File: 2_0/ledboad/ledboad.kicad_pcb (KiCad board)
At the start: 4 copper layers, 100 x 32 mm, 297 parts, among them J1 USB_C_Receptacle_USB2.0, Q10 CJX3139K, Q11 CJX3139K, Q12 CJX3139K, Q13 CJX3139K, Q14 CJX3139K, Q15 CJX3139K, Q16 CJX3139K, Q9 CJX3139K, SW2 TS-1088-AR02016, U2 74HC138PW,118

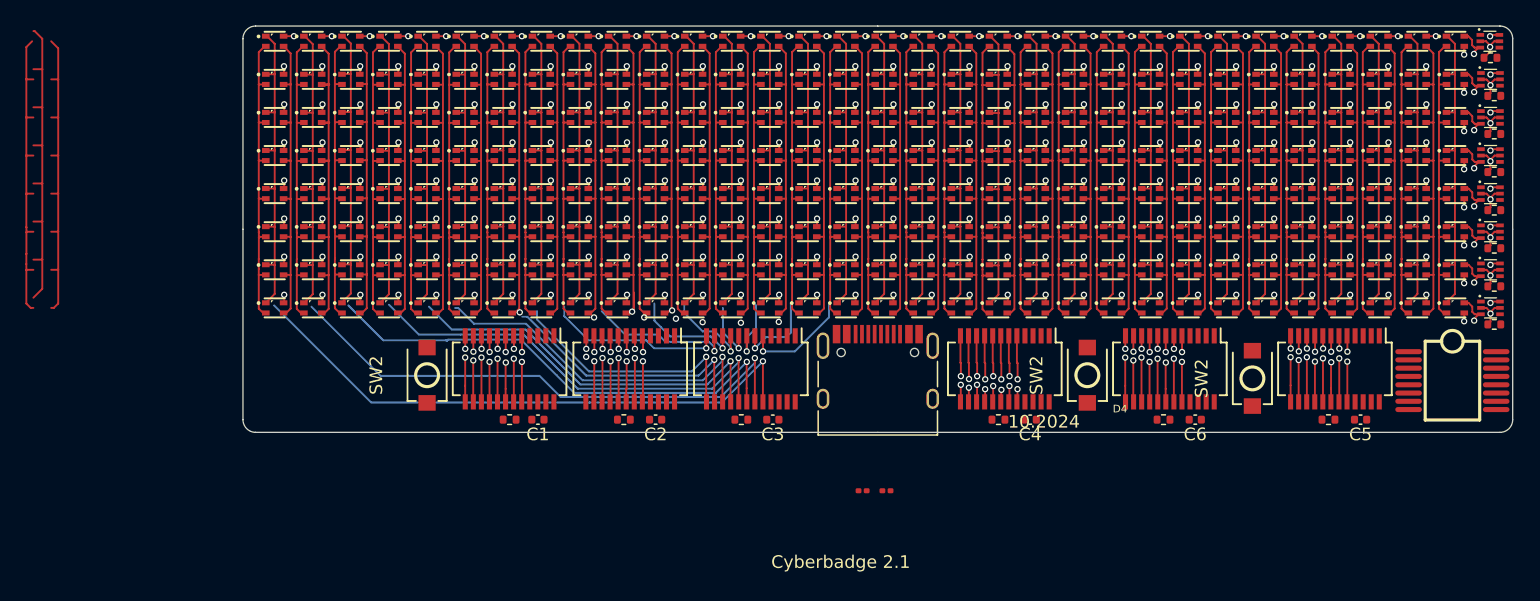
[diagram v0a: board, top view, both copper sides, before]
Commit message: work on ledboard
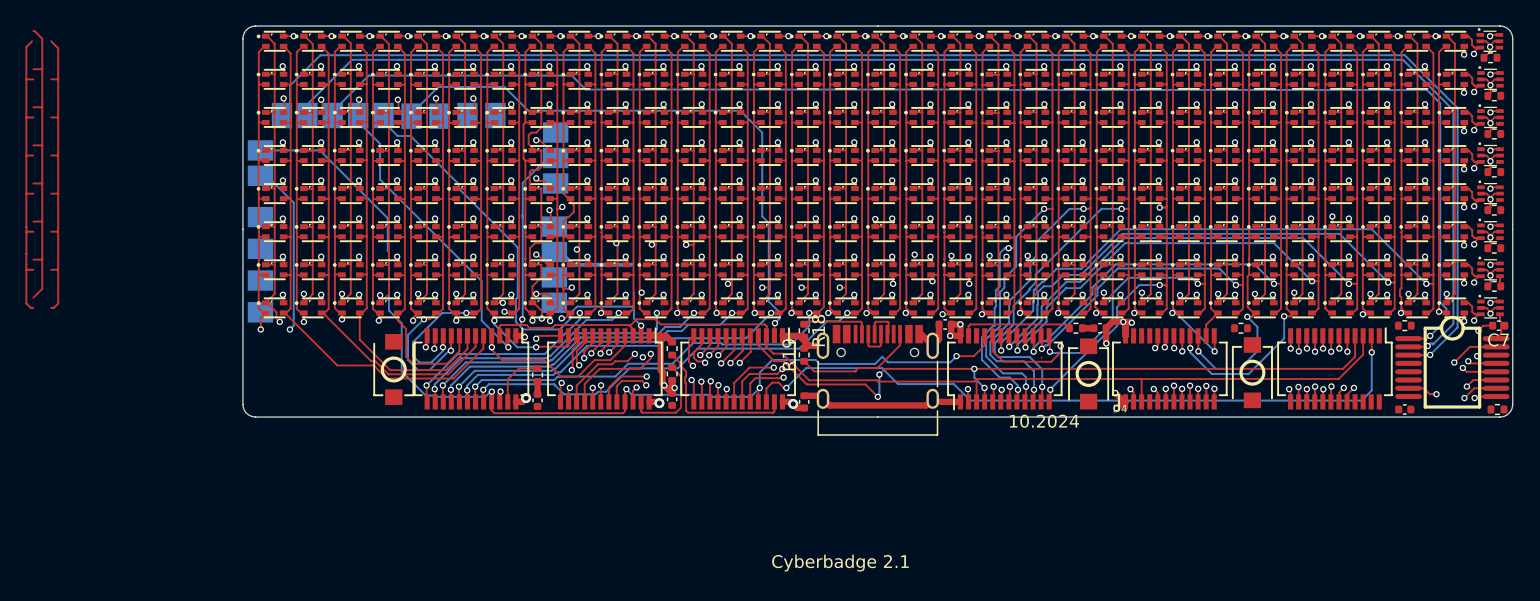
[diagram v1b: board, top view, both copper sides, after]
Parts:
- removed the SW2 at (54.5, 47.5)
- removed the SW2 at (119.5, 47.8)
- added C7: 470n, Capacitor_SMD:C_0402_1005Metric, F.Cu at (138.9, 43.6)
- added SW1: TS-1088-AR02016, easyeda2kicad:SW-SMD_L3.9-W3.0-P4.45, F.Cu at (119.5, 47.3)
- added SW3: TS-1088-AR02016, easyeda2kicad:SW-SMD_L3.9-W3.0-P4.45, F.Cu at (51.9, 47.0)
- added U1: ~, Critbit_lib:pilkbrain2, B.Cu at (53.4, 38.8)
- R18, R19: footprint Resistor_SMD:R_0201_0603Metric -> Resistor_SMD:R_0402_1005Metric
- moved C5 33.6 mm to (95.3, 43.5)
- moved C6 16.5 mm to (131.5, 50.2), turned to 0 degrees
- moved R18 14.2 mm to (84.2, 44.0), turned to -90 degrees
- moved R19 11.6 mm to (84.2, 45.9), turned to 90 degrees
- moved R9 9.53 mm to (131.5, 43.6)
- moved R11 9.44 mm to (118.6, 43.8)
- moved R13 9.44 mm to (105.6, 43.8)
- moved C4 9.06 mm to (107.5, 43.8)
- moved R10 7.81 mm to (73.8, 45.4), turned to 90 degrees
- moved R24 6.70 mm to (138.8, 50.2)
- moved R12 5.23 mm to (73.8, 47.4), turned to -90 degrees
- moved R14 4.15 mm to (63.2, 47.5), turned to -90 degrees
- moved RU6 3.00 mm to (58.0, 47.0)
- moved C3 2.84 mm to (84.2, 49.6), turned to 90 degrees
- moved C2 2.06 mm to (73.8, 49.4), turned to 90 degrees
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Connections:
- RU1 pad 10: /COL_R26 -> /COL_R21
- RU1 pad 11: /COL_R25 -> /COL_R22
- RU1 pad 12: /COL_R24 -> /COL_R23
- RU1 pad 13: /COL_R23 -> /COL_R24
- RU1 pad 14: /COL_R22 -> /COL_R25
- RU1 pad 15: /COL_R21 -> /COL_R26
- RU1 pad 16: /COL_R20 -> /COL_R27
- RU1 pad 17: /COL_R19 -> /COL_R28
- RU1 pad 18: /COL_R18 -> /COL_R29
- RU1 pad 19: /COL_R17 -> /COL_R30
- RU1 pad 2: /DAT_R -> Net-(RU1-SDI)
- RU1 pad 20: /COL_R16 -> /COL_R31
- RU1 pad 22: Net-(RU1-SDO) -> unconnected-(RU1-SDO-Pad22)
- RU1 pad 5: /COL_R31 -> /COL_R16
- RU1 pad 6: /COL_R30 -> /COL_R17
- RU1 pad 7: /COL_R29 -> /COL_R18
- RU1 pad 8: /COL_R28 -> /COL_R19
- RU1 pad 9: /COL_R27 -> /COL_R20
- RU2 pad 10: /COL_R10 -> /COL_R5
- RU2 pad 11: /COL_R9 -> /COL_R6
- RU2 pad 12: /COL_R8 -> /COL_R7
- RU2 pad 13: /COL_R7 -> /COL_R8
- RU2 pad 14: /COL_R6 -> /COL_R9
- RU2 pad 15: /COL_R5 -> /COL_R10
- RU2 pad 16: /COL_R4 -> /COL_R11
- RU2 pad 17: /COL_R3 -> /COL_R12
- RU2 pad 18: /COL_R2 -> /COL_R13
- RU2 pad 19: /COL_R1 -> /COL_R14
- RU2 pad 2: Net-(RU1-SDO) -> /DAT_R
- RU2 pad 20: /COL_R0 -> /COL_R15
- RU2 pad 22: unconnected-(RU2-SDO-Pad22) -> Net-(RU1-SDI)
- RU2 pad 5: /COL_R15 -> /COL_R0
- RU2 pad 6: /COL_R14 -> /COL_R1
- RU2 pad 7: /COL_R13 -> /COL_R2
- RU2 pad 8: /COL_R12 -> /COL_R3
- RU2 pad 9: /COL_R11 -> /COL_R4
- RU3 pad 10: /COL_G26 -> /COL_G21
- RU3 pad 11: /COL_G25 -> /COL_G22
- RU3 pad 12: /COL_G24 -> /COL_G23
- RU3 pad 13: /COL_G23 -> /COL_G24
- RU3 pad 14: /COL_G22 -> /COL_G25
- RU3 pad 15: /COL_G21 -> /COL_G26
- RU3 pad 16: /COL_G20 -> /COL_G27
- RU3 pad 17: /COL_G19 -> /COL_G28
- RU3 pad 18: /COL_G18 -> /COL_G29
- RU3 pad 19: /COL_G17 -> /COL_G30
- RU3 pad 2: /DAT_G -> Net-(RU3-SDI)
- RU3 pad 20: /COL_G16 -> /COL_G31
- RU3 pad 22: Net-(RU3-SDO) -> unconnected-(RU3-SDO-Pad22)
- RU3 pad 5: /COL_G31 -> /COL_G16
- RU3 pad 6: /COL_G30 -> /COL_G17
- RU3 pad 7: /COL_G29 -> /COL_G18
- RU3 pad 8: /COL_G28 -> /COL_G19
- RU3 pad 9: /COL_G27 -> /COL_G20
- RU4 pad 10: /COL_G10 -> /COL_G5
- RU4 pad 11: /COL_G9 -> /COL_G6
- RU4 pad 12: /COL_G8 -> /COL_G7
- RU4 pad 13: /COL_G7 -> /COL_G8
- RU4 pad 14: /COL_G6 -> /COL_G9
- RU4 pad 15: /COL_G5 -> /COL_G10
- RU4 pad 16: /COL_G4 -> /COL_G11
- RU4 pad 17: /COL_G3 -> /COL_G12
- RU4 pad 18: /COL_G2 -> /COL_G13
- RU4 pad 19: /COL_G1 -> /COL_G14
- RU4 pad 2: Net-(RU3-SDO) -> /DAT_G
- RU4 pad 20: /COL_G0 -> /COL_G15
- RU4 pad 22: unconnected-(RU4-SDO-Pad22) -> Net-(RU3-SDI)
- RU4 pad 5: /COL_G15 -> /COL_G0
- RU4 pad 6: /COL_G14 -> /COL_G1
- RU4 pad 7: /COL_G13 -> /COL_G2
- RU4 pad 8: /COL_G12 -> /COL_G3
- RU4 pad 9: /COL_G11 -> /COL_G4
- RU5 pad 10: /COL_B26 -> /COL_B21
- RU5 pad 11: /COL_B25 -> /COL_B22
- RU5 pad 12: /COL_B24 -> /COL_B23
- RU5 pad 13: /COL_B23 -> /COL_B24
- RU5 pad 14: /COL_B22 -> /COL_B25
- RU5 pad 15: /COL_B21 -> /COL_B26
- RU5 pad 16: /COL_B20 -> /COL_B27
- RU5 pad 17: /COL_B19 -> /COL_B28
- RU5 pad 18: /COL_B18 -> /COL_B29
- RU5 pad 19: /COL_B17 -> /COL_B30
- RU5 pad 2: /DAT_B -> Net-(RU5-SDI)
- RU5 pad 20: /COL_B16 -> /COL_B31
- RU5 pad 22: Net-(RU5-SDO) -> unconnected-(RU5-SDO-Pad22)
- RU5 pad 5: /COL_B31 -> /COL_B16
- RU5 pad 6: /COL_B30 -> /COL_B17
- RU5 pad 7: /COL_B29 -> /COL_B18
- RU5 pad 8: /COL_B28 -> /COL_B19
- RU5 pad 9: /COL_B27 -> /COL_B20
- RU6 pad 10: /COL_B10 -> /COL_B5
- RU6 pad 11: /COL_B9 -> /COL_B6
- RU6 pad 12: /COL_B8 -> /COL_B7
- RU6 pad 13: /COL_B7 -> /COL_B8
- RU6 pad 14: /COL_B6 -> /COL_B9
- RU6 pad 15: /COL_B5 -> /COL_B10
- RU6 pad 16: /COL_B4 -> /COL_B11
- RU6 pad 17: /ROW_7 -> /COL_B12
- RU6 pad 18: /COL_B2 -> /COL_B13
- RU6 pad 19: /COL_B1 -> /COL_B14
- RU6 pad 2: Net-(RU5-SDO) -> /DAT_B
- RU6 pad 20: /COL_B0 -> /COL_B15
- RU6 pad 22: unconnected-(RU6-SDO-Pad22) -> Net-(RU5-SDI)
- RU6 pad 5: /COL_B15 -> /COL_B0
- RU6 pad 6: /COL_B14 -> /COL_B1
- RU6 pad 7: /COL_B13 -> /COL_B2
- RU6 pad 8: /COL_B12 -> /COL_B3
- RU6 pad 9: /COL_B11 -> /COL_B4
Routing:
- net /MATRIX_C: track 0.00 -> 119.8 mm, vias 0 -> 1
- net /MATRIX_B: track 0.00 -> 116.0 mm, vias 0 -> 1
- net /MATRIX_A: track 0.00 -> 110.9 mm, vias 0 -> 1
- net /LAT: track 0.00 -> 101.9 mm, vias 0 -> 6
- net /SCLK: track 0.00 -> 93.5 mm, vias 0 -> 1
- net /OE: track 0.00 -> 79.6 mm, vias 0 -> 4
- net Net-(RU1-SDI): track 0.00 -> 55.4 mm, vias 0 -> 2
- net VDD: track 0.00 -> 52.6 mm, vias 0 -> 8
- net /DAT_R: track 0.00 -> 47.4 mm, vias 0 -> 1
- net /COL_R16: track 29.0 -> 75.6 mm, vias 1 -> 2
- net Net-(RU3-SDI): track 0.00 -> 45.1 mm, vias 0 -> 2
- net /COL_R17: track 29.2 -> 72.3 mm, vias 1 -> 2
- net /COL_B31: track 29.7 -> 70.8 mm
- net Net-(RU5-SDI): track 0.00 -> 39.8 mm, vias 0 -> 2
- net /COL_R18: track 28.9 -> 68.1 mm, vias 1 -> 2
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- added copper zone on In2.Cu, net GND
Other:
- board size 100 x 32 mm -> 100 x 30.8 mm

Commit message: before oder
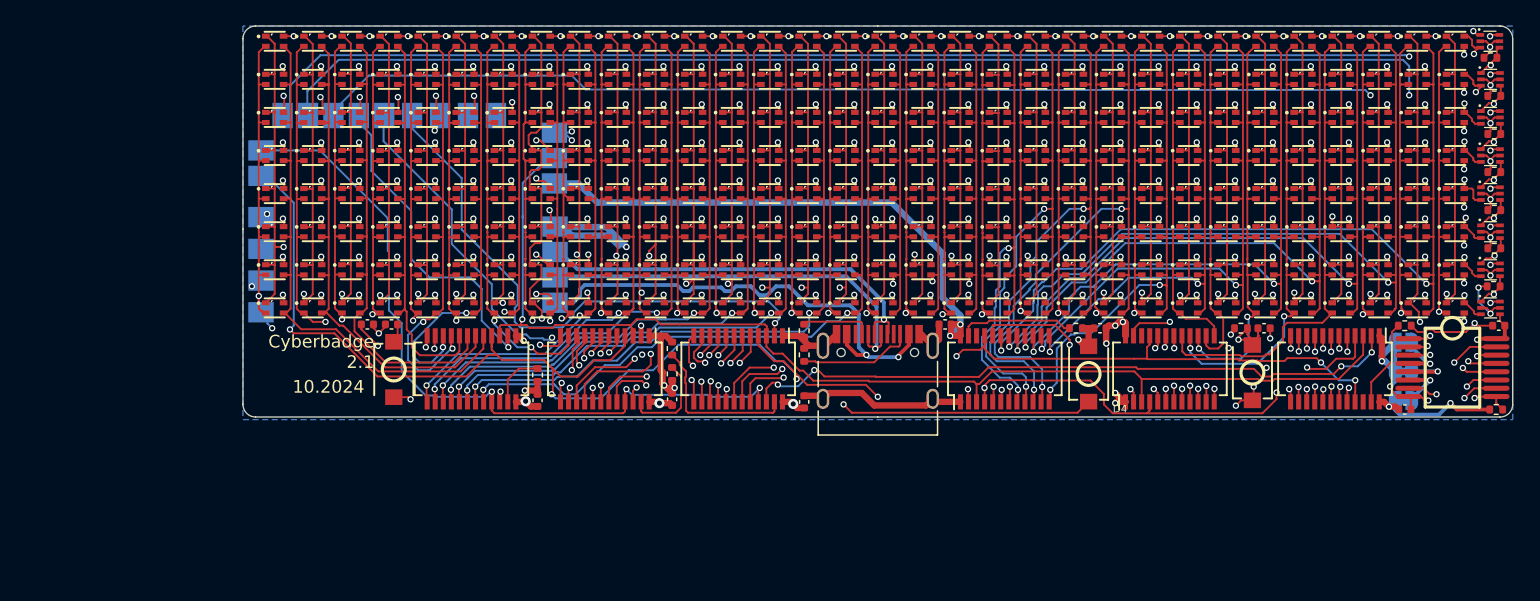
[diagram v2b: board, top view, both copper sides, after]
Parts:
- added C10: 470n, Capacitor_SMD:C_0402_1005Metric, F.Cu at (51.7, 43.5)
- added C8: 470n, Capacitor_SMD:C_0402_1005Metric, F.Cu at (49.8, 43.5)
- added C9: 470n, Capacitor_SMD:C_0402_1005Metric, F.Cu at (120.4, 43.8)
- added JP1: SB, Jumper:SolderJumper-2_P1.3mm_Bridged_RoundedPad1.0x1.5mm, B.Cu at (131.4, 44.9)
- added JP2: SB, Jumper:SolderJumper-2_P1.3mm_Bridged_RoundedPad1.0x1.5mm, B.Cu at (131.4, 47.2)
- added JP3: SB, Jumper:SolderJumper-2_P1.3mm_Bridged_RoundedPad1.0x1.5mm, B.Cu at (131.4, 49.5)
- moved R24 9.70 mm to (138.5, 40.5)
- moved R23 9.70 mm to (138.7, 50.2), turned to 0 degrees
- moved U1 0.35 mm to (53.0, 38.8)
- turned SW1 to 90 degrees
- turned SW2 to 90 degrees
- turned SW3 to -90 degrees
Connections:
- SW1 pad 1: unconnected-(SW1-Pad1) -> /B1
- SW1 pad 2: unconnected-(SW1-Pad2) -> GND
- SW2 pad 1: unconnected-(SW2-Pad1) -> /B2
- SW2 pad 2: unconnected-(SW2-Pad2) -> GND
- SW3 pad 2: unconnected-(SW3-Pad2) -> GND
- U1 pad 5V: unconnected-(U1-5V_IN-Pad5V) -> VBUS
- U1 pad DM: unconnected-(U1-USB_DM-PadDM) -> /DM
- U1 pad DP: unconnected-(U1-USB_DP-PadDP) -> /DP
- U1 pad SCL: unconnected-(U1-PadSCL) -> /B2
- U1 pad SDA: unconnected-(U1-PadSDA) -> /B1
- U2 pad 4: unconnected-(U2-~{E1}-Pad4) -> Net-(JP1-A)
- U2 pad 5: unconnected-(U2-~{E2}-Pad5) -> Net-(JP2-A)
- U2 pad 6: unconnected-(U2-E3-Pad6) -> Net-(JP3-A)
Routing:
- net /B1: track 0.00 -> 88.4 mm, vias 0 -> 5
- net VDD: track 52.6 -> 127.8 mm, vias 8 -> 19
- net /B2: track 0.00 -> 73.7 mm, vias 0 -> 3
- net GND: track 35.4 -> 89.1 mm, vias 6 -> 19
- net VBUS: track 0.00 -> 38.0 mm, vias 0 -> 2
- net /OE: track 79.6 -> 113.8 mm, vias 4 -> 6
- net /DM: track 2.85 -> 32.7 mm, vias 0 -> 1
- net /DP: track 3.00 -> 32.4 mm, vias 0 -> 1
- net /COL_R0: track 98.7 -> 69.5 mm
- net /LAT: track 101.9 -> 129.8 mm, vias 6 -> 7
- net /COL_B0: track 69.7 -> 44.3 mm
- net /COL_G0: track 83.4 -> 59.3 mm
- net /COL_G28: track 26.2 -> 40.2 mm, vias 1 -> 0
- net Net-(RU3-REXT): track 0.00 -> 9.47 mm, vias 0 -> 2
- net unconnected-(U1-USB_DP-PadDP): track 6.99 -> 0.00 mm
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- added copper zone on B.Cu, net VDD
